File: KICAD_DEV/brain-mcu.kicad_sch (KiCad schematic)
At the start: 21 parts, among them SW1 SW_Push, SW2 SW_Push, U1 STM32H743VITx, Y1 8 MHz, Y2 32.768 KHz

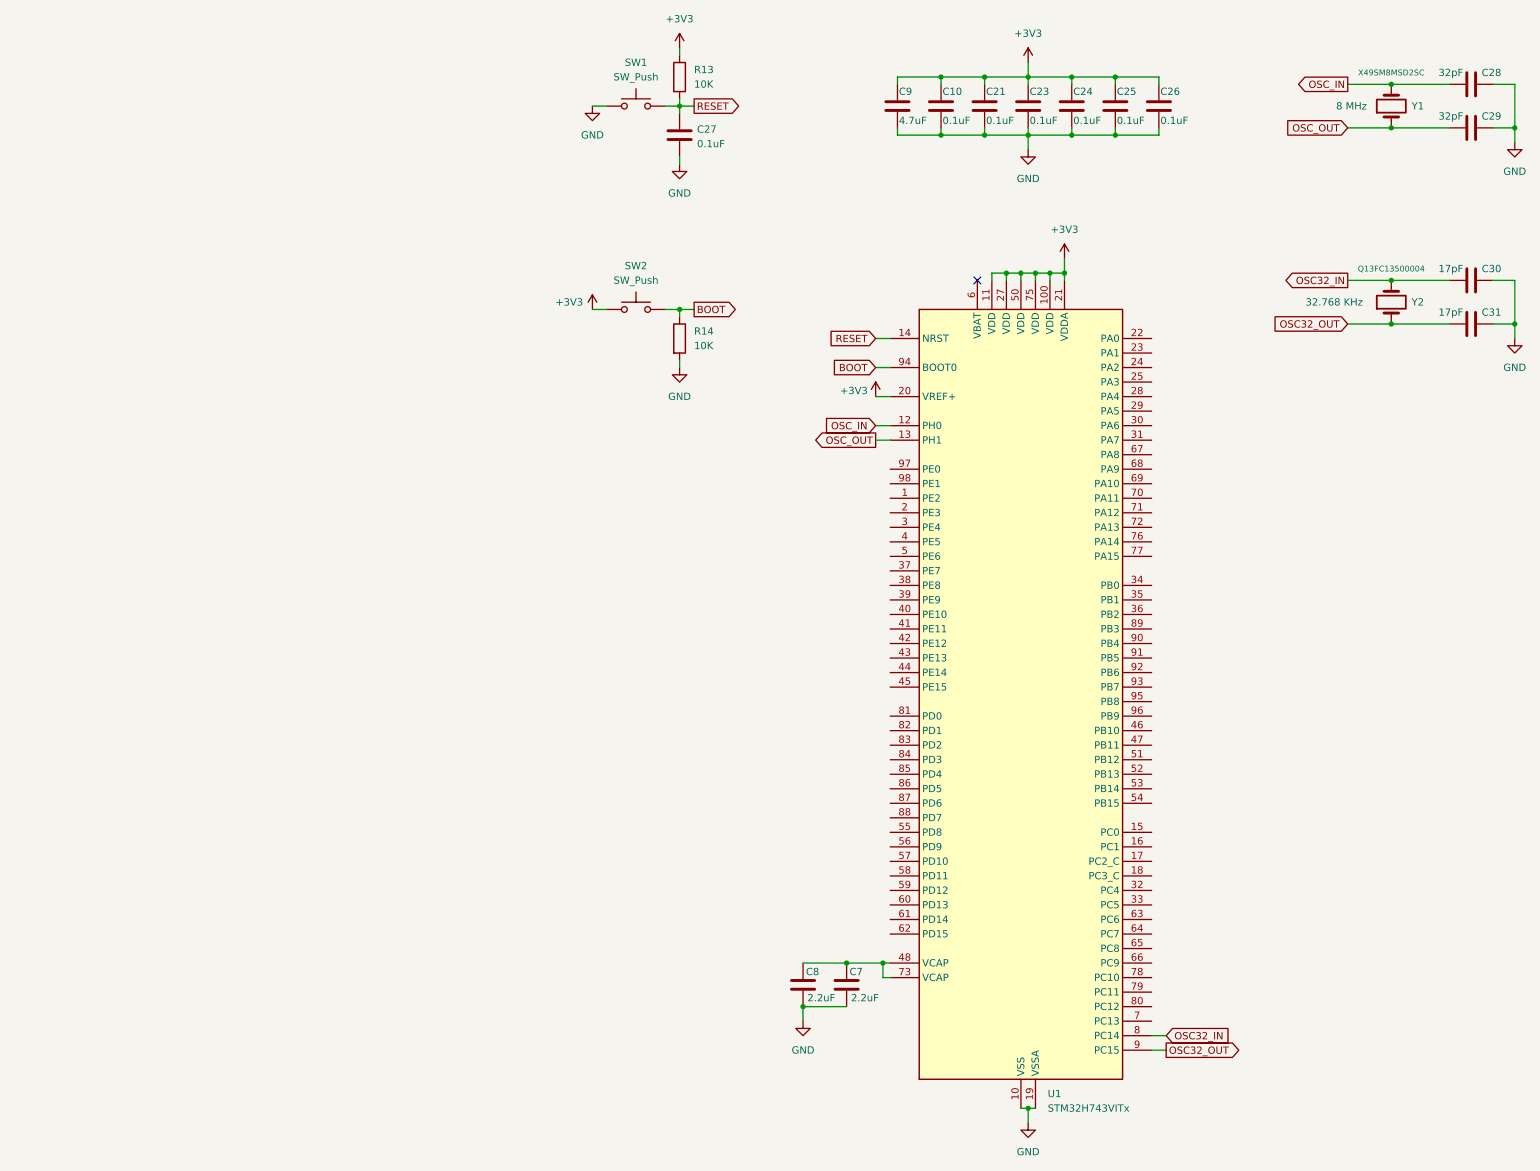
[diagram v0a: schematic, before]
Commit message: cleaning stuff up!
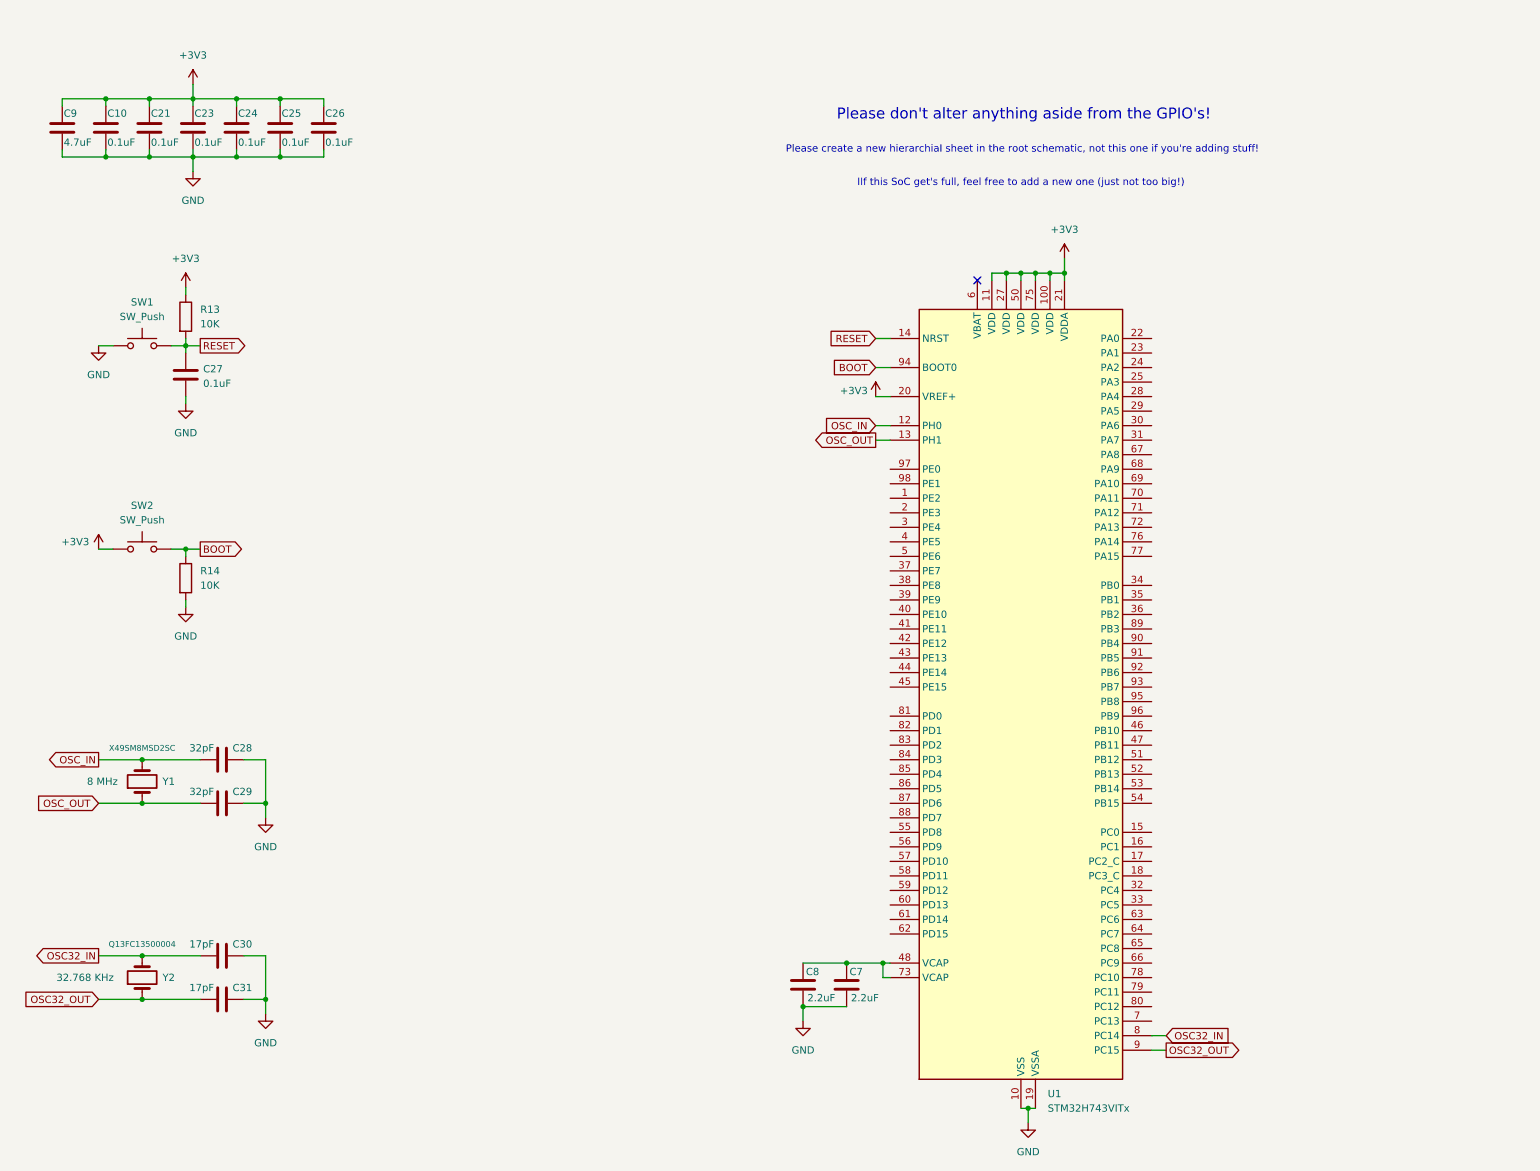
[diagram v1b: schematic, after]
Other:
- note added: "IIf this SoC get's full, feel free to add a new one (just not too big!)"
- note added: "Please create a new hierarchial sheet in the root schematic, not this one if you're adding stuff!"
- note added: "Please don't alter anything aside from the GPIO's!"
- moved on the sheet: C10, C21, C23, C24, C25, C26, C27, C28, C29, C30, C31, C9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
